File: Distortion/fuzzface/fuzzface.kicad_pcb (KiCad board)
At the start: 2 copper layers, 52 x 28.5 mm, 13 parts, among them J1 Conn_01x04_Female, Q1 AC128, Q2 AC128

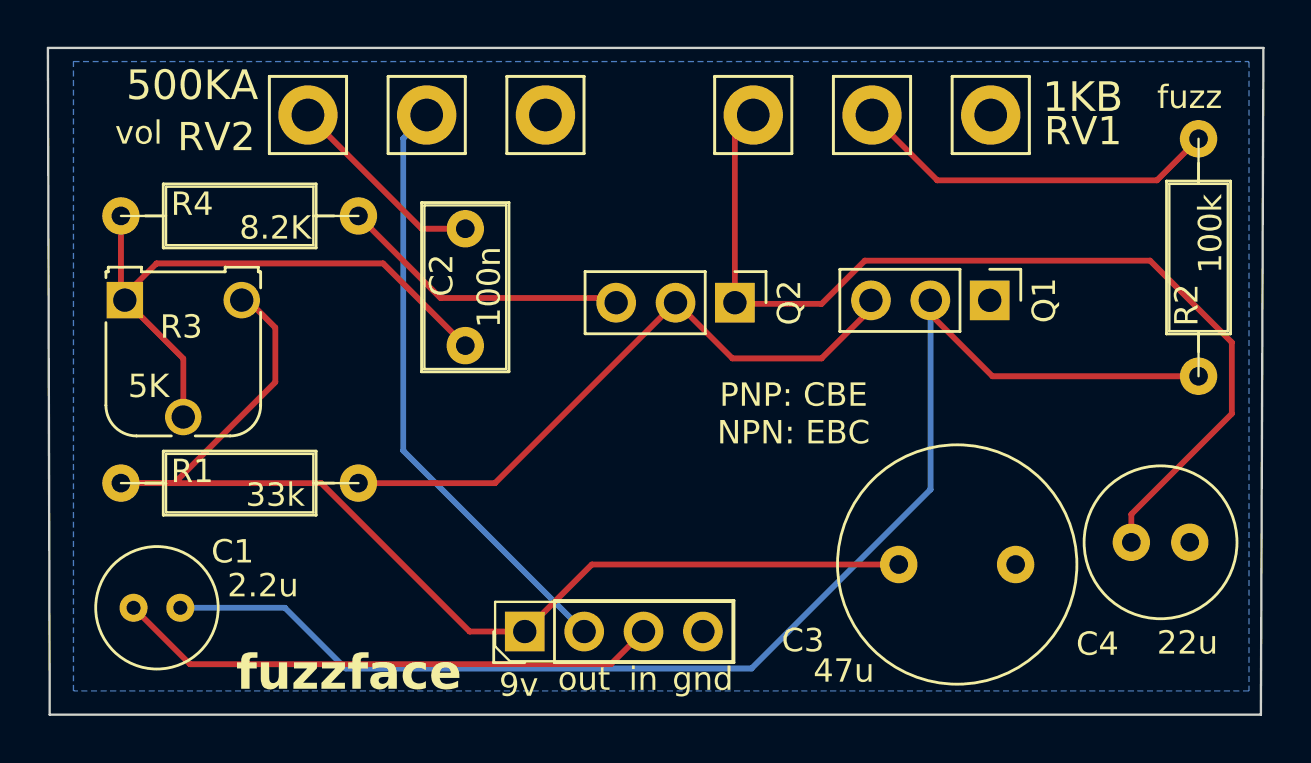
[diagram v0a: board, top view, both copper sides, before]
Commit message: added ejfuzzface
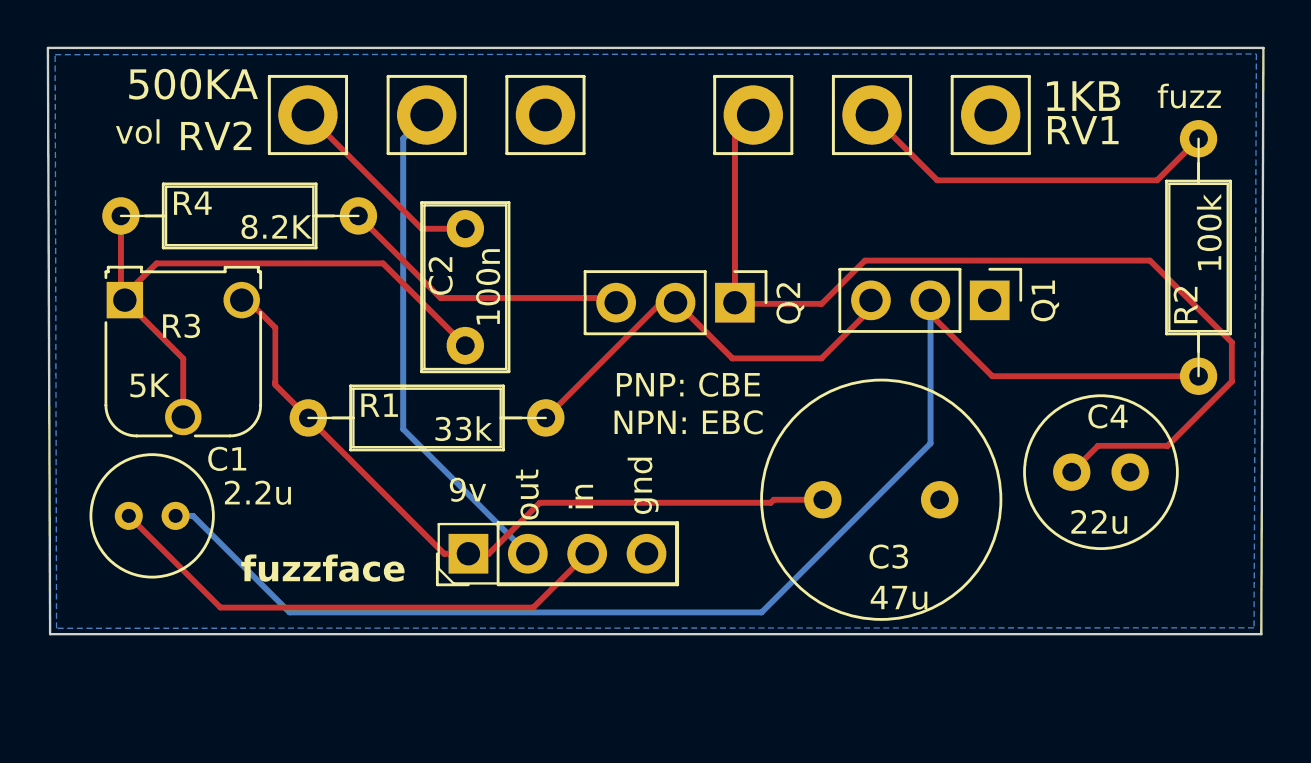
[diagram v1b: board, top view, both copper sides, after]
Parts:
- moved R1 8.49 mm to (121.3, 115.8)
- moved C3 4.27 mm to (133.2, 119.3)
- moved J1 4.11 mm to (118.0, 121.6)
- moved C4 3.94 mm to (143.8, 118.2)
- moved C1 3.94 mm to (103.5, 120.0)
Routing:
- net -9Vor9V: track 50.1 -> 31.7 mm
- net Net-(Q1-C): track 26.9 -> 17.8 mm
- net OUT: track 25.7 -> 21.4 mm
- net Net-(Q1-B): track 56.4 -> 55.1 mm
- net IN: track 23.4 -> 22.2 mm
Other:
- board size 52 x 28.5 mm -> 52 x 25.1 mm
- board text added: "+"
